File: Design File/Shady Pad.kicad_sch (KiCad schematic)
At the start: 28 parts, among them J2 Conn_01x04_Pin, SW1 SW_Push, SW2 SW_Push, SW3 SW_Push, SW4 SW_Push, SW5 SW_Push, SW6 SW_Push, SW7 RotaryEncoder_Switch, SW8 SW_Push, SW9 SW_Push, U1 MOUDLE-SEEEDUINO-XIAO

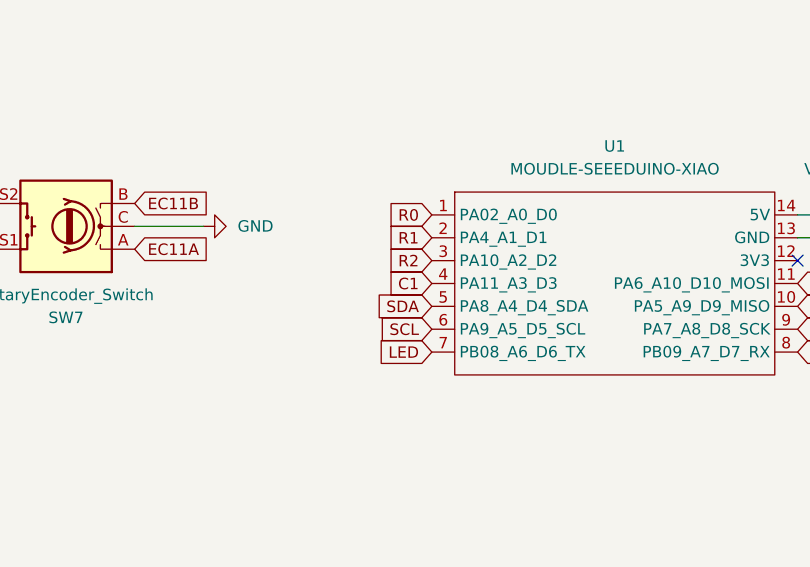
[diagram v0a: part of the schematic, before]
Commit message: kk
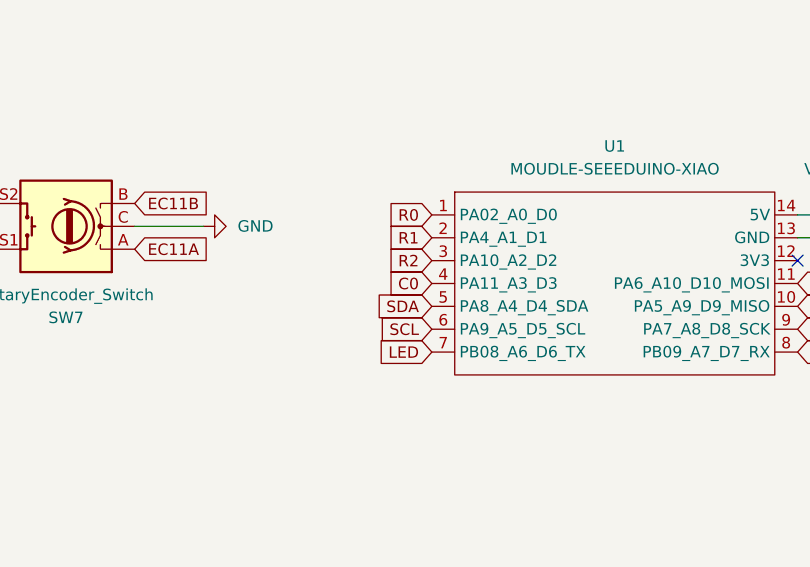
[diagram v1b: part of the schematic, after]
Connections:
- net C0: now also U1.4 (PA11_A3_D3)
- net C1: no longer U1.4 (PA11_A3_D3)
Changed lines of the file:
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@@
 		)
 	)
-	(global_label "C1"
+	(global_label "C0"
 		(shape input)
 		(at 198.12 85.09 180)
